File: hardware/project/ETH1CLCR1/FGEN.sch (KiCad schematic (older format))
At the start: 81 parts, among them U1401 ECS-3225SMV-500-GP-TR, U1402 REF192, U1403 74AHCT1G08, U1404 AD5689BRUZ, U1405 AD9835, U1406 TL072, U1407 DG419LDY, U1408 AD5453YRMZ, U1409 LT1468, U1410 LT1468, U1411 LT1468

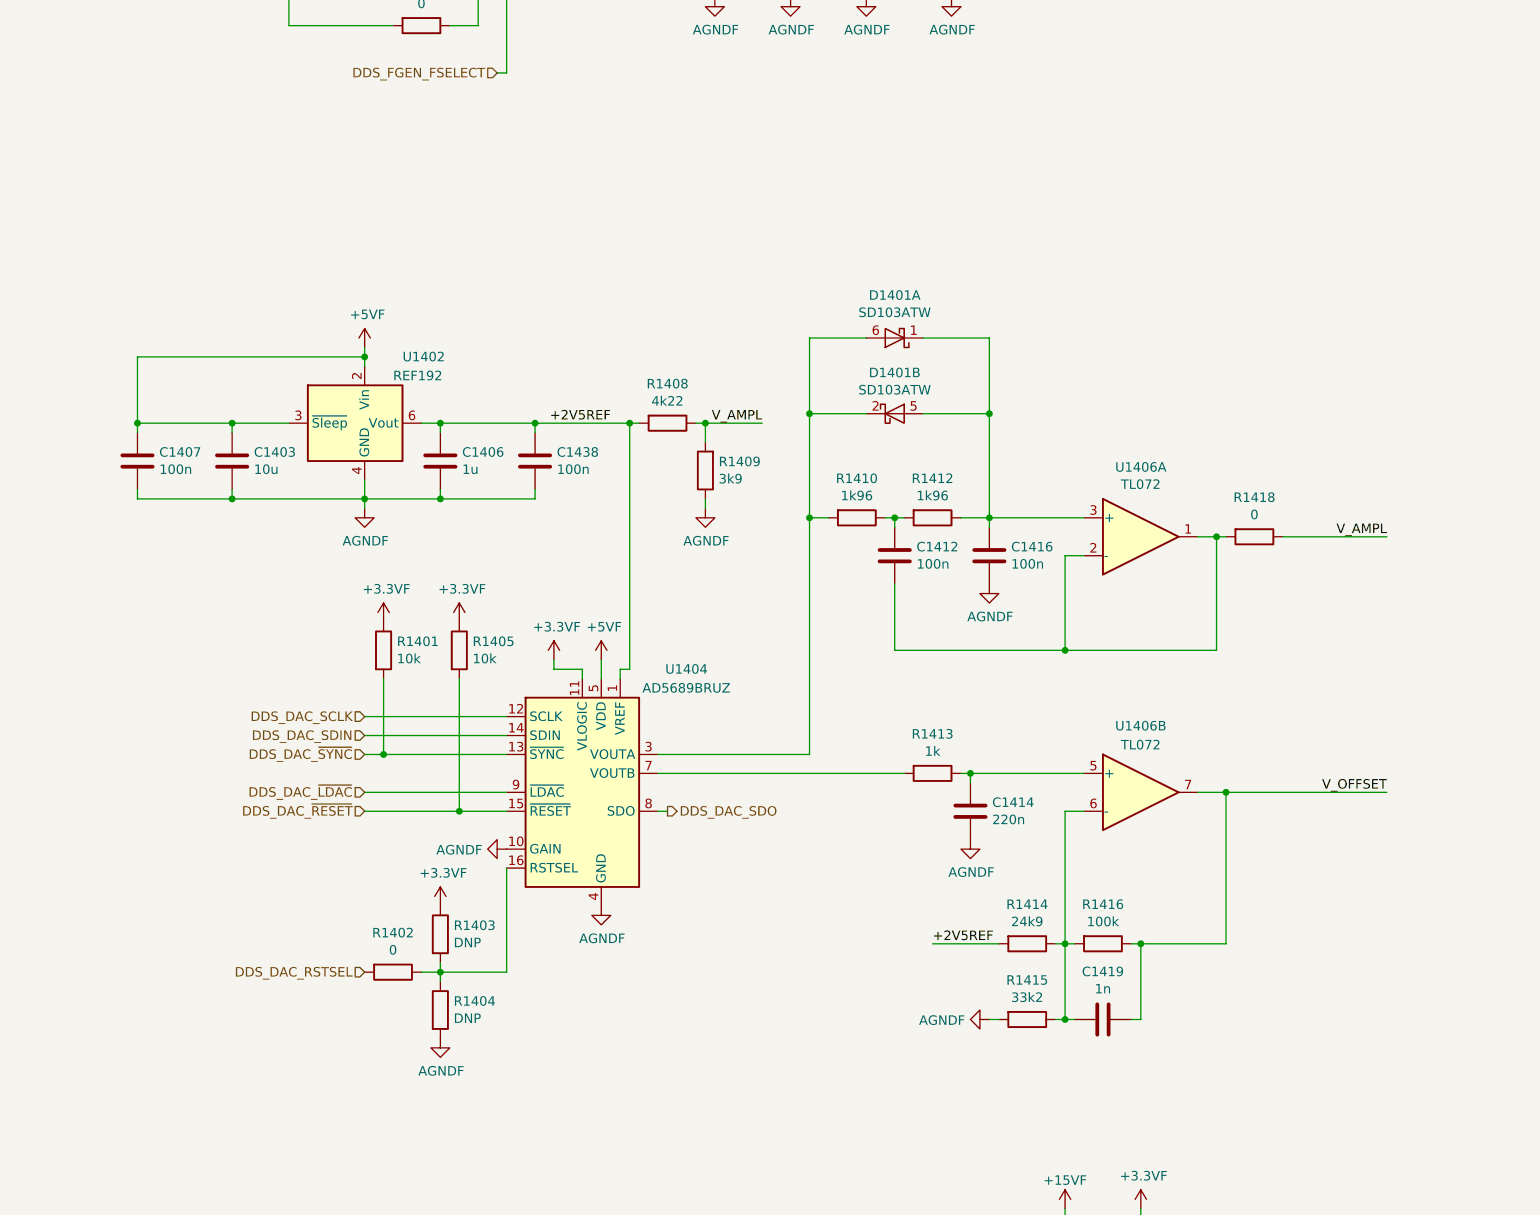
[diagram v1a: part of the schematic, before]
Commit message: PCB done.
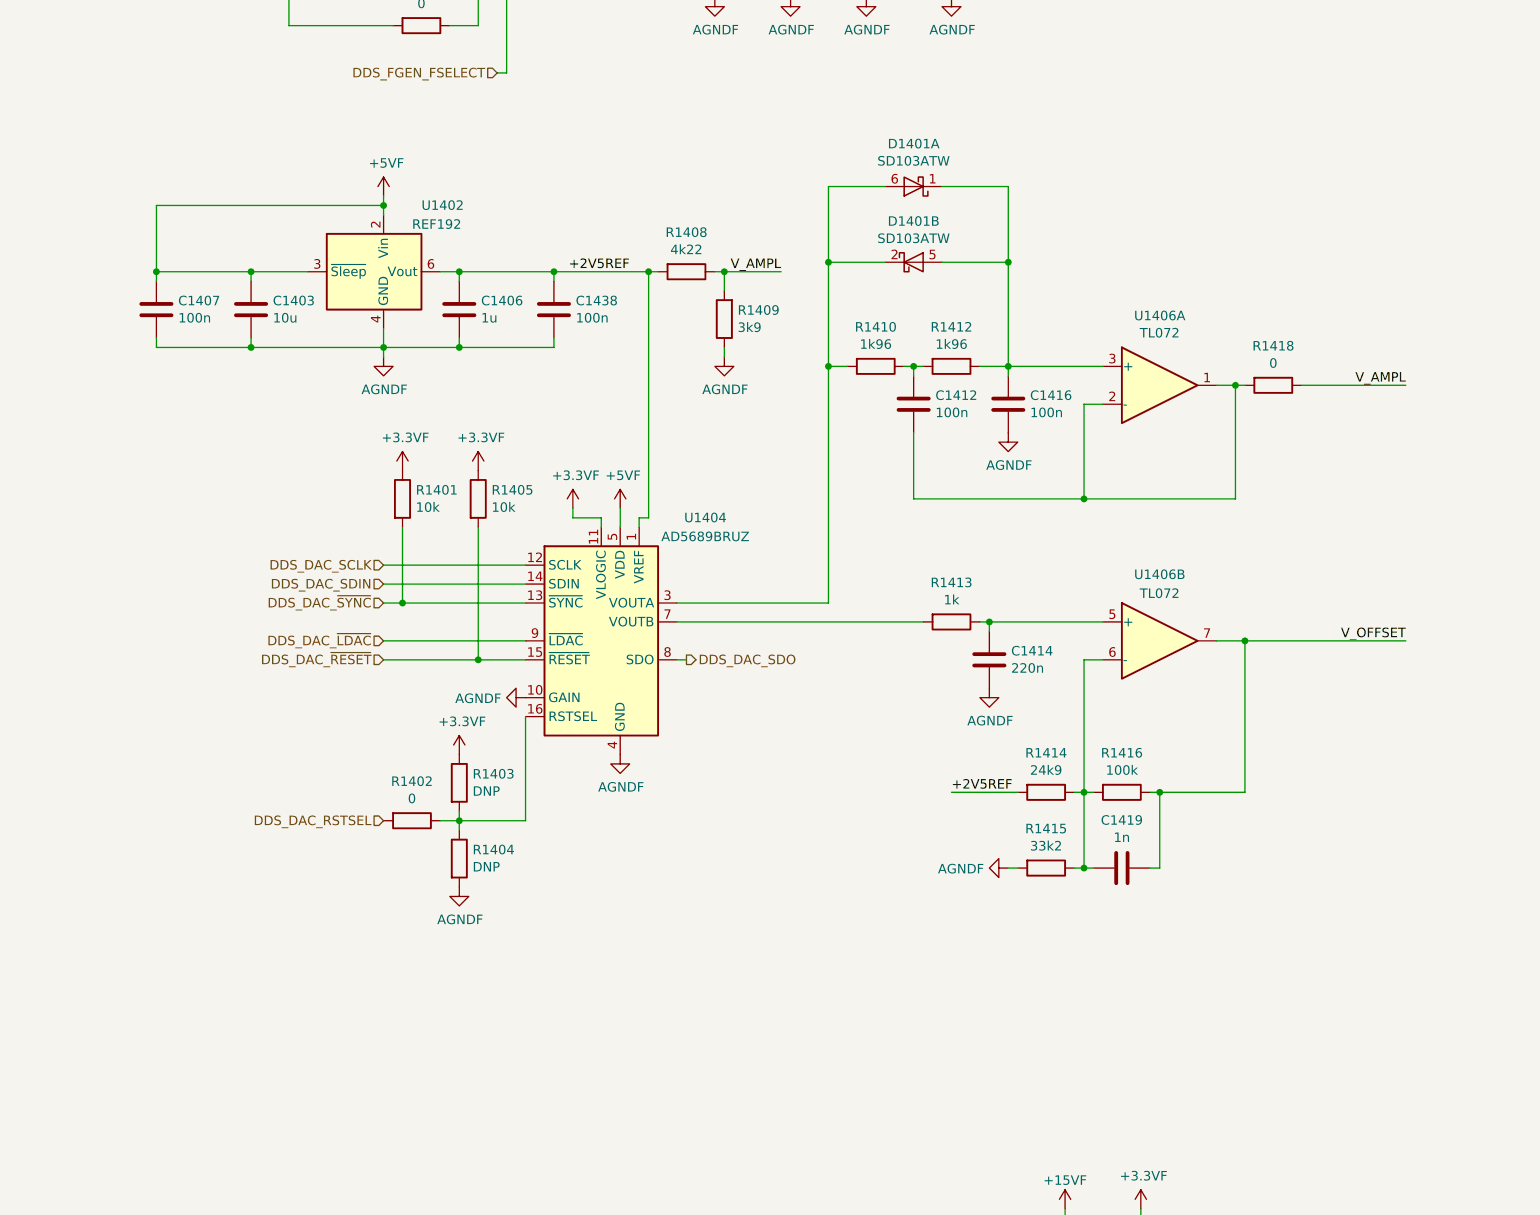
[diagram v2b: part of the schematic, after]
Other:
- moved on the sheet: C1403, C1406, C1407, C1412, C1414, C1416, C1419, C1438, D1401A, D1401B, R1401, R1402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
